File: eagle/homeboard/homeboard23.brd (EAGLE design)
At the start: 94 x 71.8 mm, 128 parts, among them IC1 XCF02S, IC2 25LC080SN, IC3 ATMEGA32U2-TQFP, Q5 BC848SMD, Q6 BC848SMD, Q7 BC848SMD, Q8 BC848SMD, T1 BSS138, T2 BC848, T3 BSS138, U1 XC3S400TQ144, X1 SCART-CLIP, X6 MINI-USB_4P-85-32004-10X, X7 DC21MMX, X8 STEREOJACK

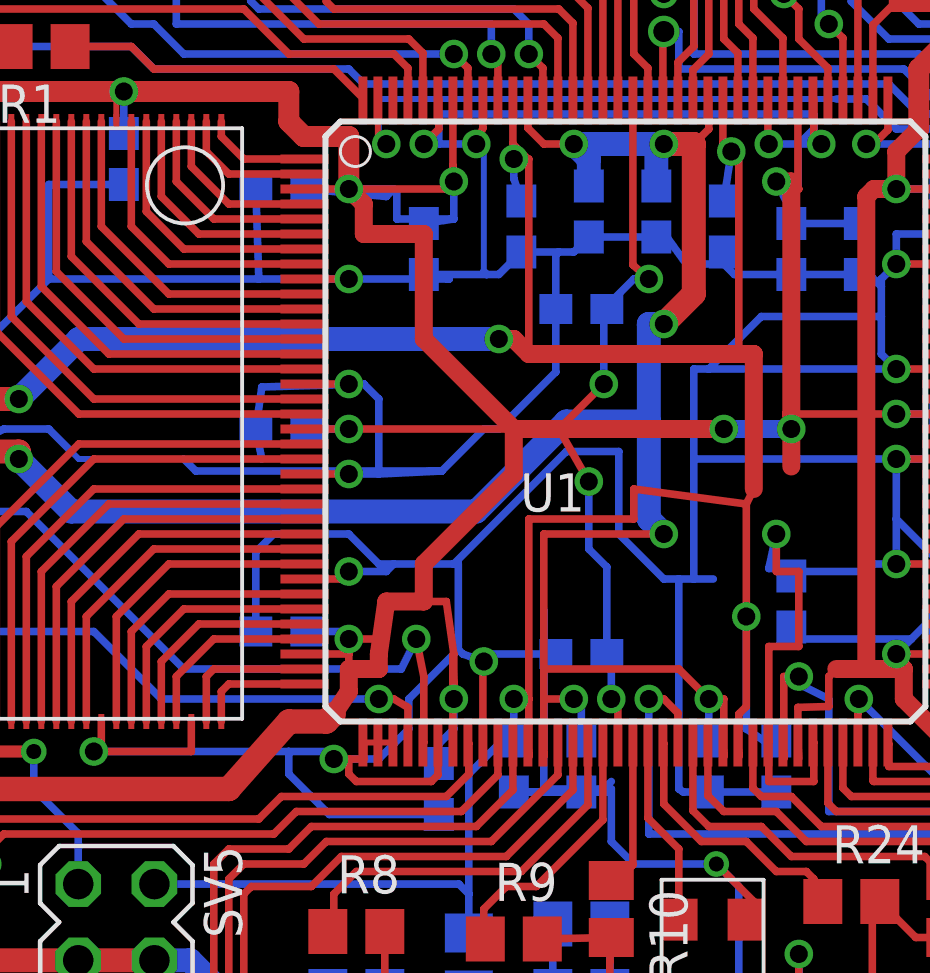
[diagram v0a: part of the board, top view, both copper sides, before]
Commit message: more
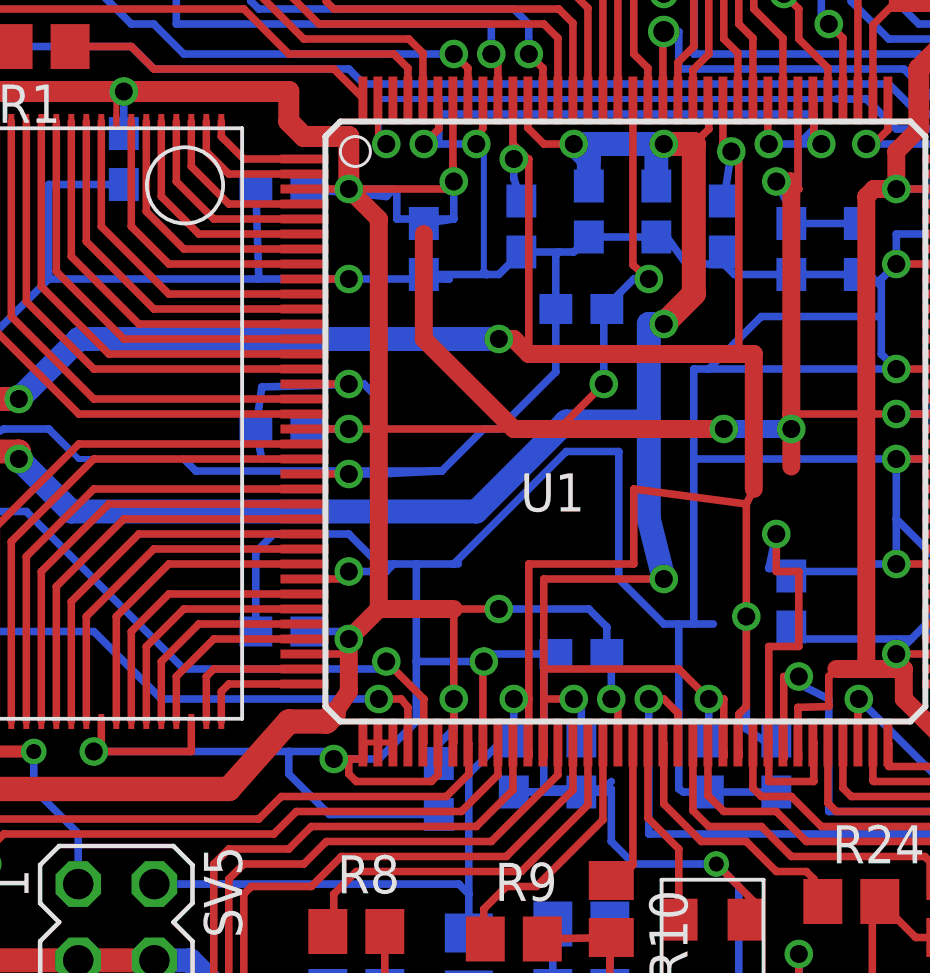
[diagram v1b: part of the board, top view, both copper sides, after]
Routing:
- net VCC: track 561.6 -> 557.5 mm
- net SD_CLK: track 23.2 -> 21.5 mm
- net GND: track 1012.8 -> 1013.5 mm
